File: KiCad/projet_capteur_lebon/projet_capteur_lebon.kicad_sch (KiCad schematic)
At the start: 16 parts, among them J1 Power, J2 Digital/PWM, J3 Analog, J4 Digital/PWM

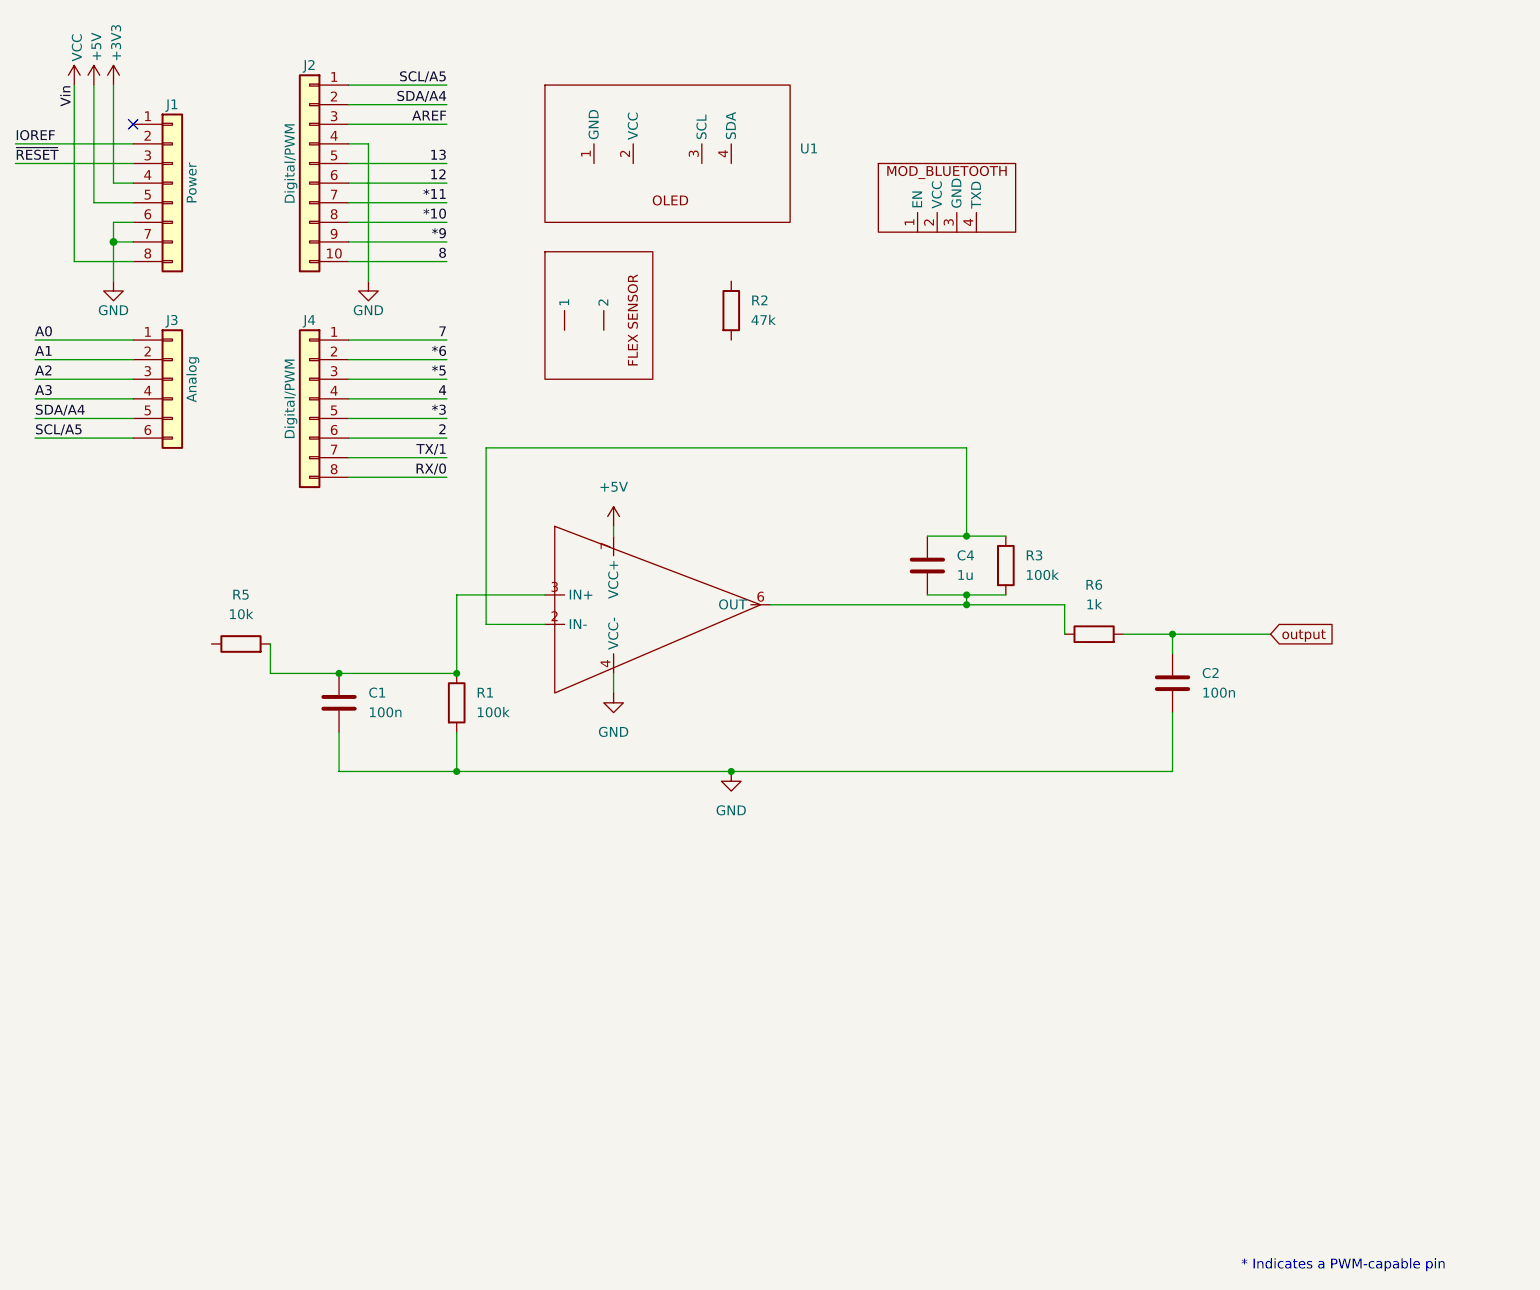
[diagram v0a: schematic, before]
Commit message: encodeur rot + verifs
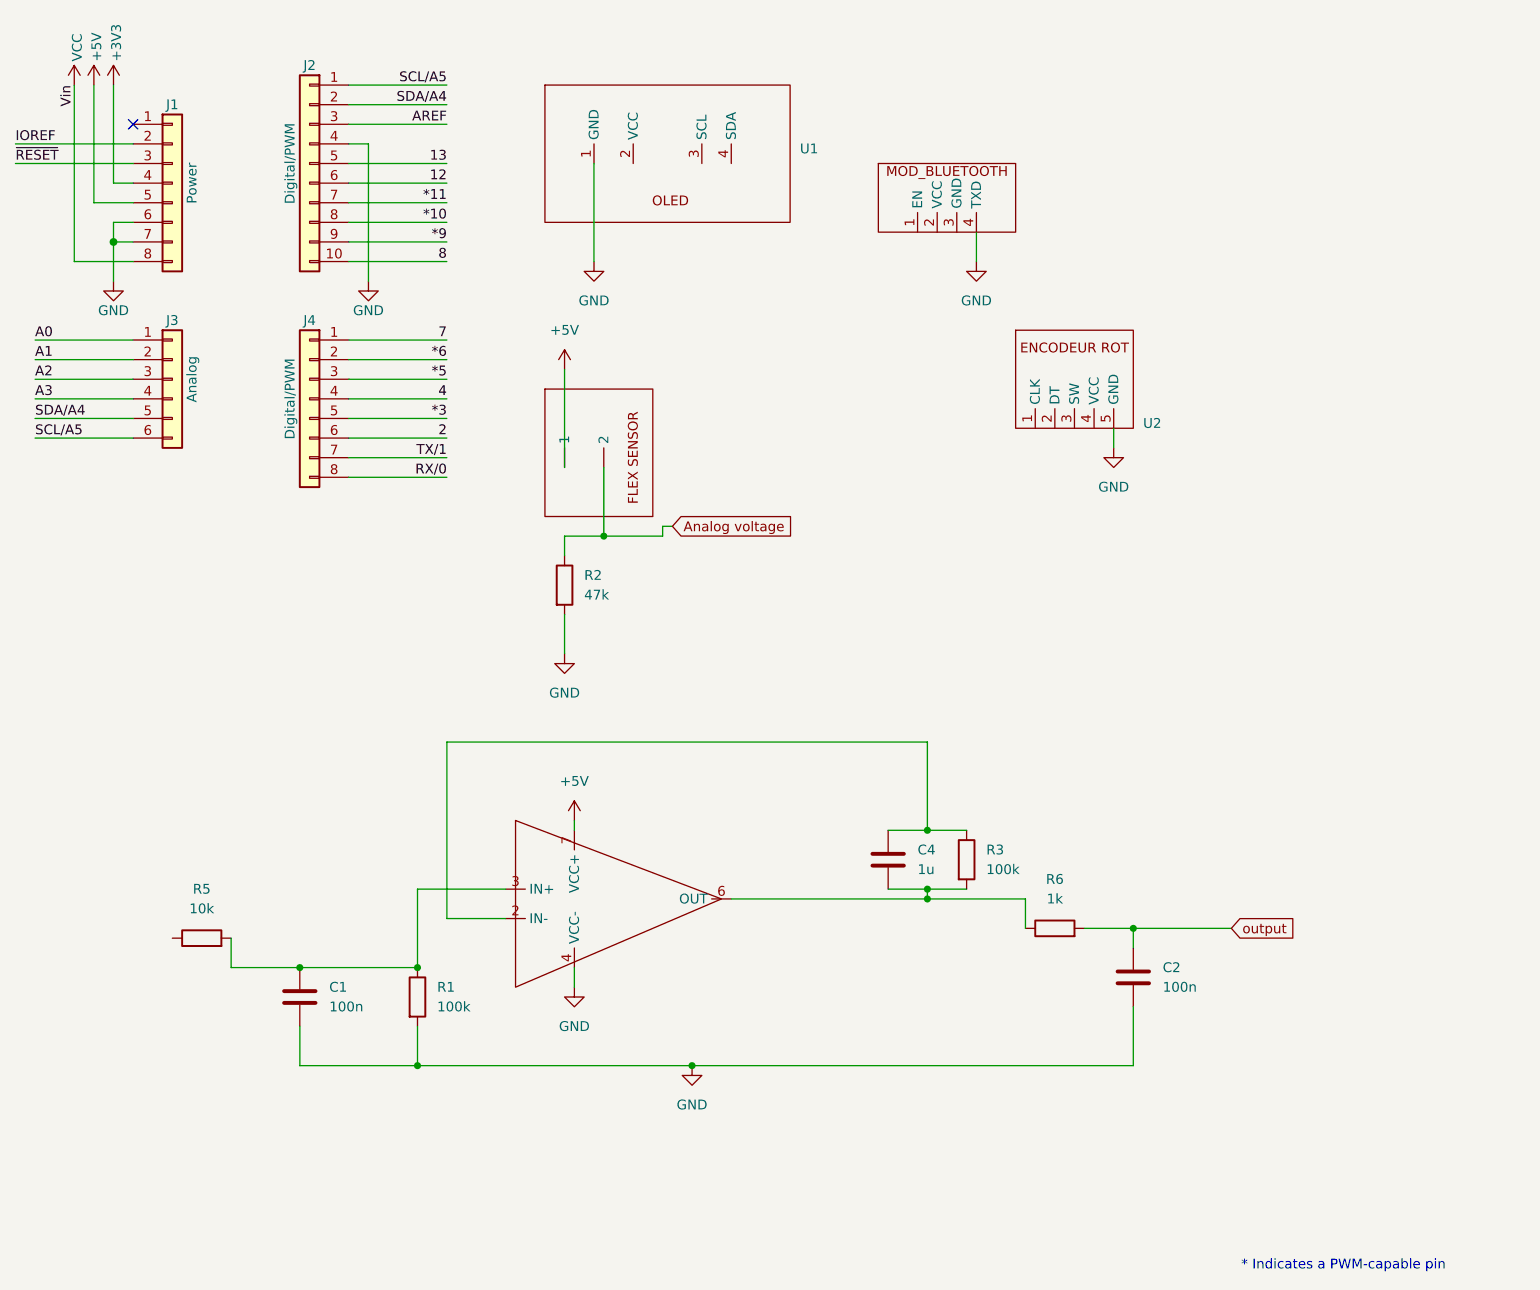
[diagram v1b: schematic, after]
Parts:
- added U2: ~, librairie_empreintes:ENCODEUR ROT, symbol librairie symboles:ENCODEUR_ROTATOIRE
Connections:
- net +5V: now also U5. (2)
- net GND: now also R2.2, U1.1 (GND), U3.4 (TXD), U2.5 (GND)
- net Analog voltage: now reaches U5. (2)
- net Analog voltage: now also R2.1
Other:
- moved on the sheet: C1, C2, C4, R1, R2, R3, R5, R6
